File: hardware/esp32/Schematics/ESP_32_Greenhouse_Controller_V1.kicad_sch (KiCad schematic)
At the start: 24 parts, among them Q1 DMP1045UQ, Q2 S8050, Q3 2N2222A, Q4 2N2222A, Q5 Mystery Transistor, T1 24 V 1 A <-- 230 V, U2 12 V OUT <-- 24 V IN, U3 3.3 V OUT <-- 24 V IN, U4 HT7550-1-SOT89, U6 DHT11

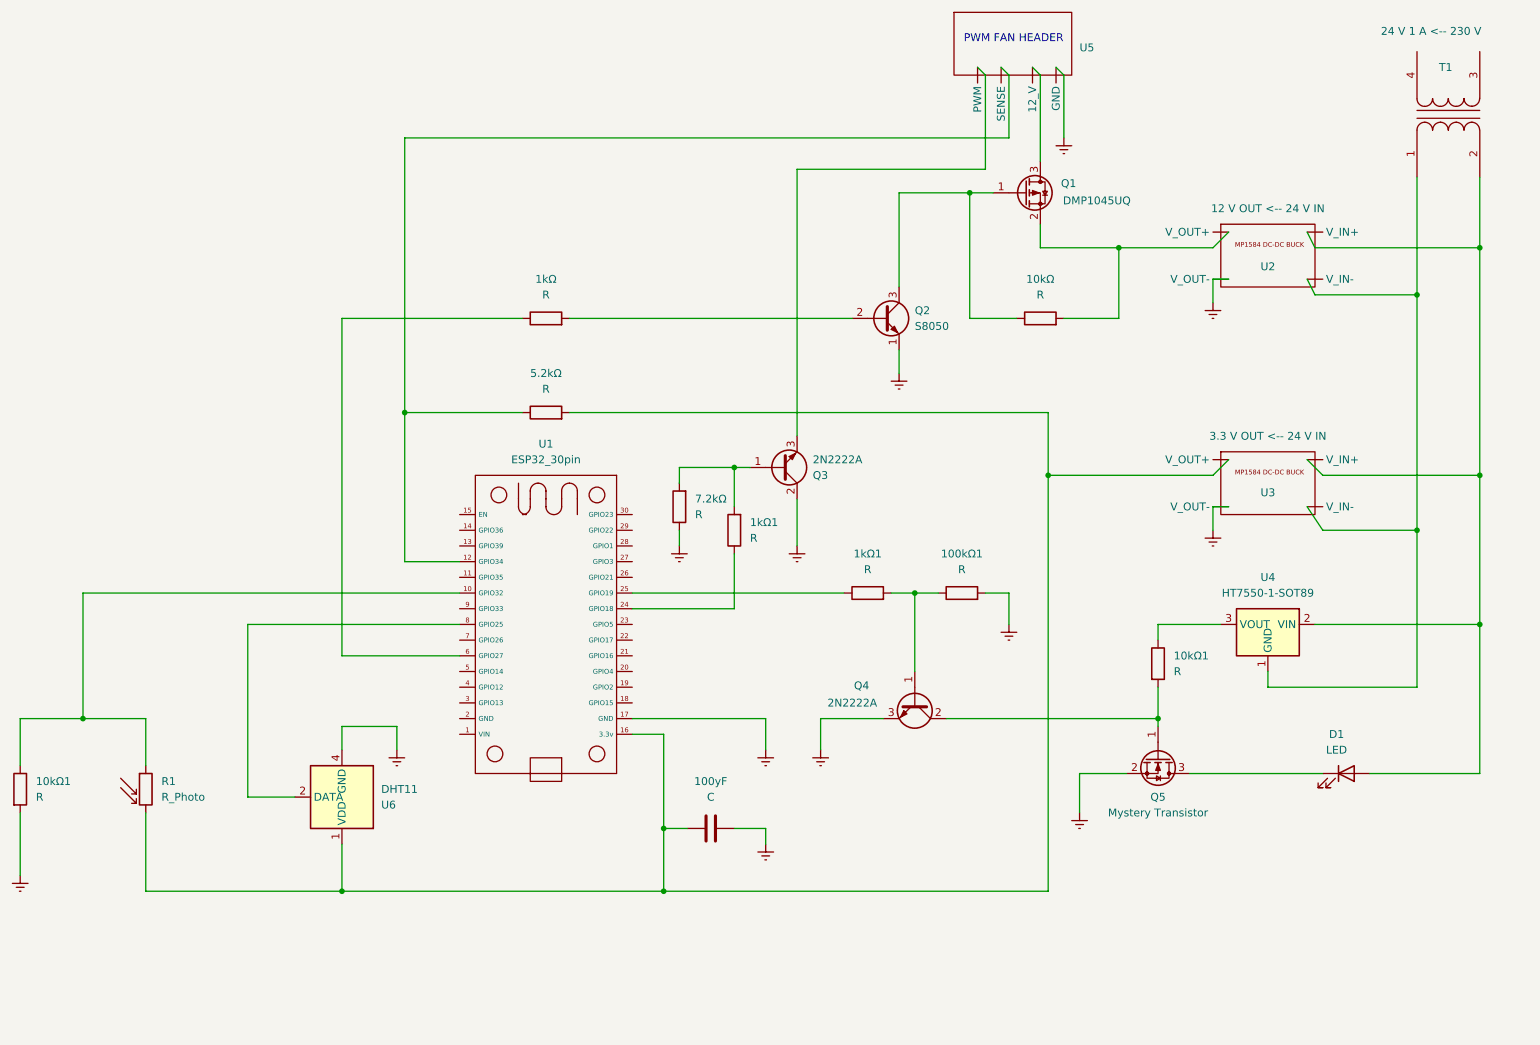
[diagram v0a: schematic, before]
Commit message: Try Try again?
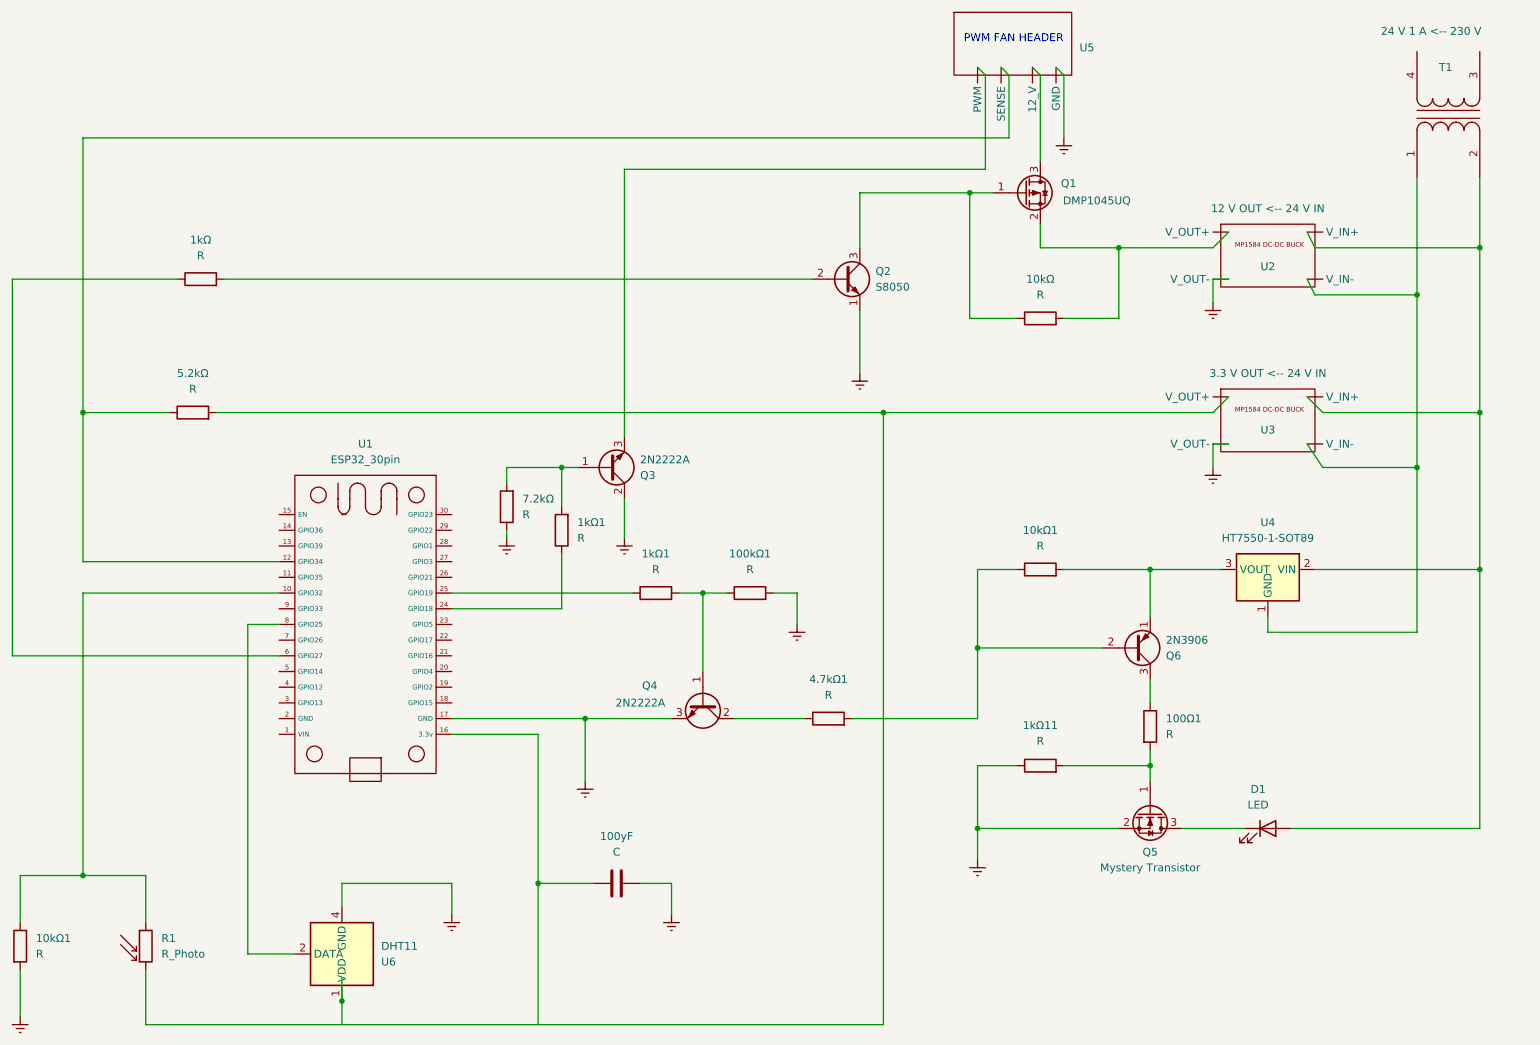
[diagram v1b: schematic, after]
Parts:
- added 10kΩ1, 1kΩ11, 4.7kΩ1: R, symbol Device:R
- added Q6: 2N3906, Package_TO_SOT_THT:TO-92_Inline, symbol Transistor_BJT:2N3906
- renumbered 10kΩ1 to 100Ω1
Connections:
- net at U3. (V_IN-): now also T1.1 (AA), U2. (V_IN-), U4.1 (GND)
- net at U4.3 (VOUT): now also 10kΩ1.2, Q6.1 (E); no longer 100Ω1.1
- net at 100Ω1.2, Q5.1 (G): now also 1kΩ11.2; no longer Q4.2 (C)
- net at Q5.2 (S): now also 1kΩ11.1
- net at U1.17 (GND): now also Q4.3 (E)
- net at U5. (GND): now also Q1.3 (D)
- new net: 5.2kΩ.2, R1.2, U3. (V_IN-)
- new net: 10kΩ1.1, 4.7kΩ1.2, Q6.2 (B)
- new net: 100Ω1.1, Q6.3 (C)
- new net: 100yF.1, U1.16 (3.3v)
- new net: 4.7kΩ1.1, Q4.2 (C)
- now unconnected: U2. (V_IN-), U6.1 (VDD)
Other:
- moved on the sheet: 100kΩ1, 100yF, 100Ω1, 10kΩ1, 1kΩ, 1kΩ1, 5.2kΩ, 7.2kΩ, D1, Q2, Q3, Q4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
